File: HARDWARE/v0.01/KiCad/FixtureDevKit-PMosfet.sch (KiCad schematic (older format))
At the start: 56 parts, among them J63 FET_0, J64 FET_4, J65 FET_1, J66 FET_5, J67 FET_2, J68 FET_6, J69 FET_3, J70 FET_7, Q10 NTF2955T1G, Q11 NTF2955T1G, Q12 NTF2955T1G, Q5 NTF2955T1G, Q6 NTF2955T1G, Q7 NTF2955T1G, Q8 NTF2955T1G, Q9 NTF2955T1G

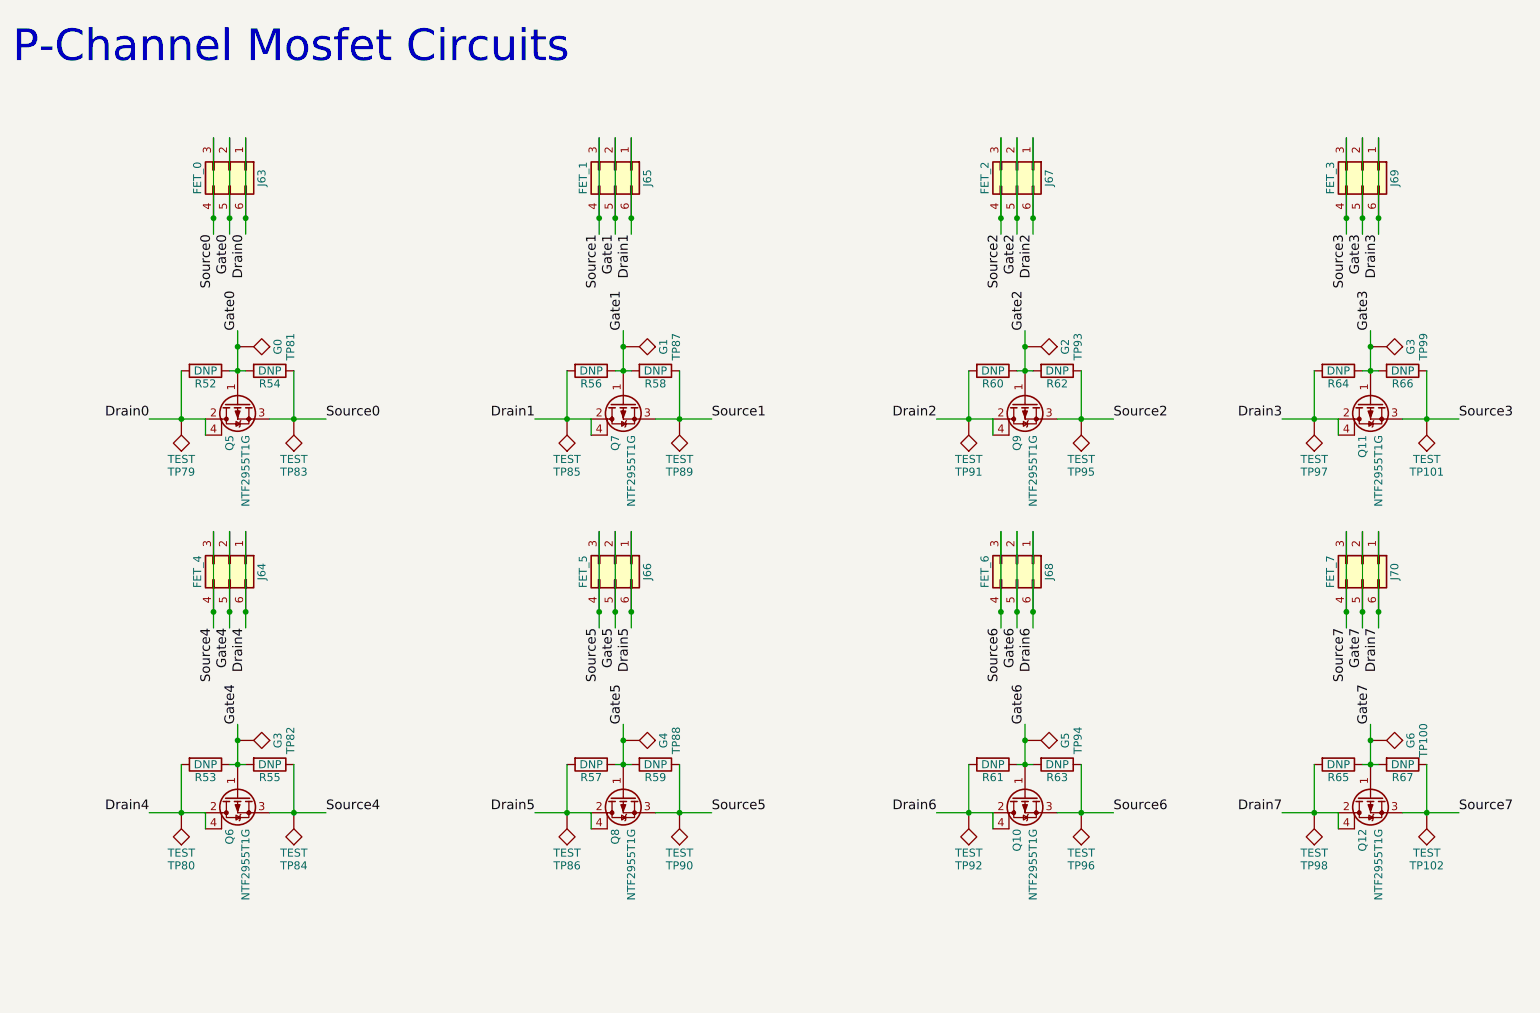
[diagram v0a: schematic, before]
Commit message: beginning pcb layout
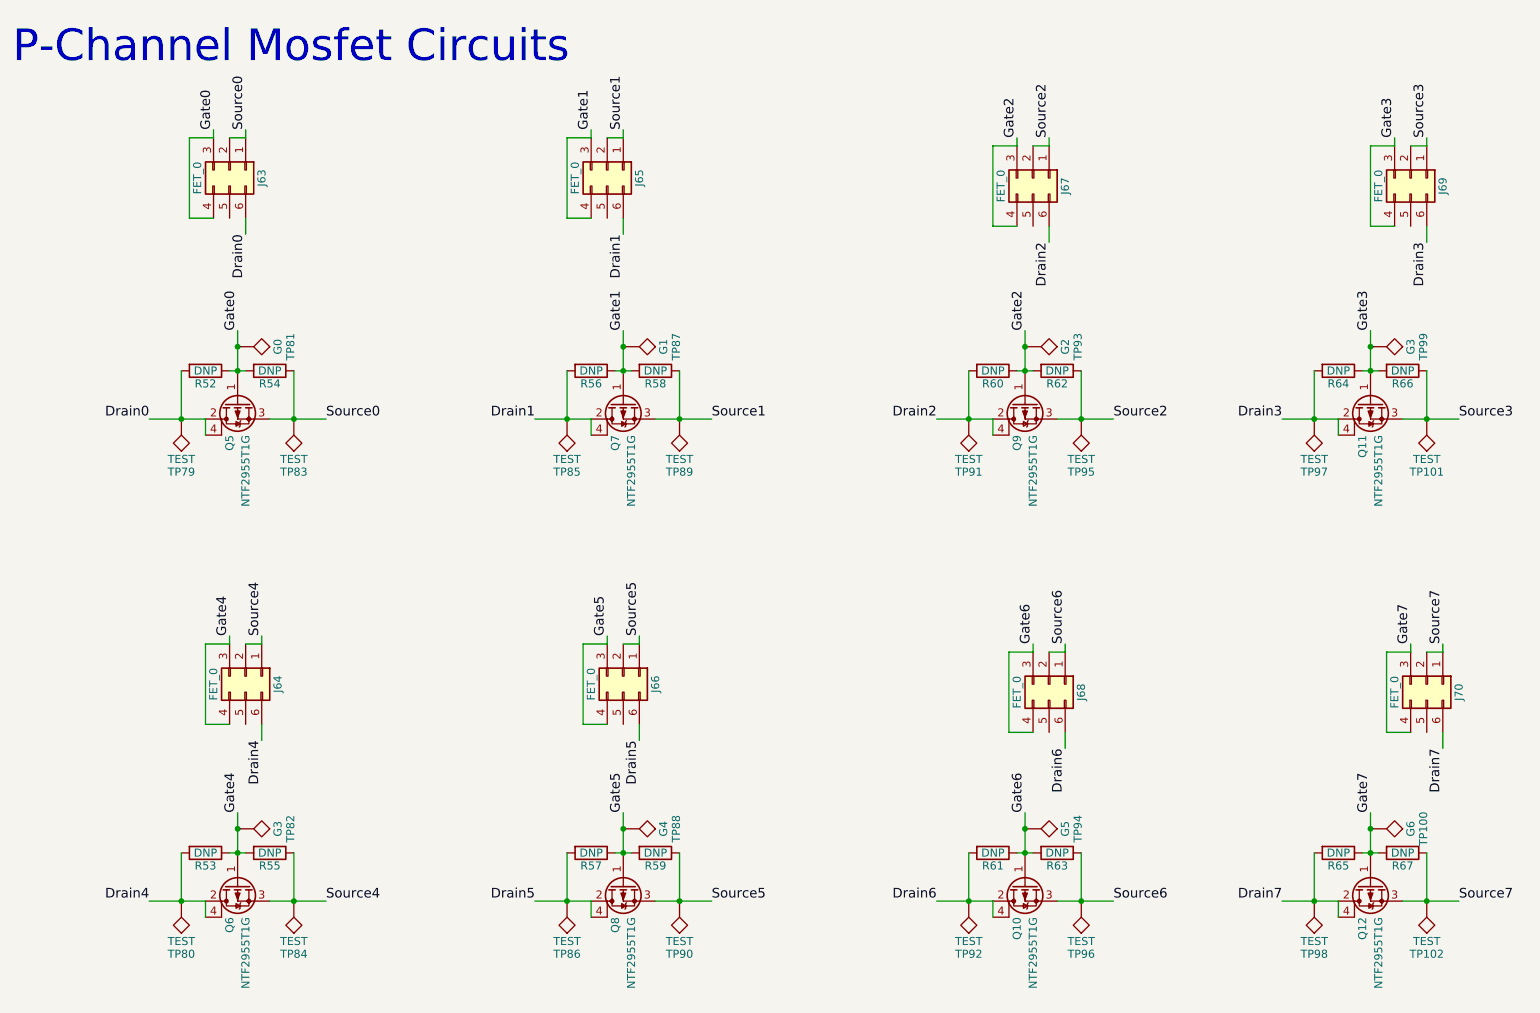
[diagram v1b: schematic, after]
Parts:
- J64: value FET_4 -> FET_0
- J65: value FET_1 -> FET_0
- J66: value FET_5 -> FET_0
- J67: value FET_2 -> FET_0
- J68: value FET_6 -> FET_0
- J69: value FET_3 -> FET_0
- J70: value FET_7 -> FET_0
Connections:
- net Drain0: no longer J63.1 (Pin_1)
- net Drain1: no longer J65.1 (Pin_1)
- net Drain2: no longer J67.1 (Pin_1)
- net Drain3: no longer J69.1 (Pin_1)
- net Drain4: no longer J64.1 (Pin_1)
- net Drain5: no longer J66.1 (Pin_1)
- net Drain6: no longer J68.1 (Pin_1)
- net Drain7: no longer J70.1 (Pin_1)
- net Gate0: now also J63.3 (Pin_3), J63.4 (Pin_4); no longer J63.2 (Pin_2), J63.5 (Pin_5)
- net Gate1: now also J65.3 (Pin_3), J65.4 (Pin_4); no longer J65.2 (Pin_2), J65.5 (Pin_5)
- net Gate2: now also J67.3 (Pin_3), J67.4 (Pin_4); no longer J67.2 (Pin_2), J67.5 (Pin_5)
- net Gate3: now also J69.3 (Pin_3), J69.4 (Pin_4); no longer J69.2 (Pin_2), J69.5 (Pin_5)
- net Gate4: now also J64.3 (Pin_3), J64.4 (Pin_4); no longer J64.2 (Pin_2), J64.5 (Pin_5)
- net Gate5: now also J66.3 (Pin_3), J66.4 (Pin_4); no longer J66.2 (Pin_2), J66.5 (Pin_5)
- net Gate6: now also J68.3 (Pin_3), J68.4 (Pin_4); no longer J68.2 (Pin_2), J68.5 (Pin_5)
- net Gate7: now also J70.3 (Pin_3), J70.4 (Pin_4); no longer J70.2 (Pin_2), J70.5 (Pin_5)
- net Source0: now also J63.1 (Pin_1), J63.2 (Pin_2); no longer J63.3 (Pin_3), J63.4 (Pin_4)
- net Source1: now also J65.1 (Pin_1), J65.2 (Pin_2); no longer J65.3 (Pin_3), J65.4 (Pin_4)
- net Source2: now also J67.1 (Pin_1), J67.2 (Pin_2); no longer J67.3 (Pin_3), J67.4 (Pin_4)
- net Source3: now also J69.1 (Pin_1), J69.2 (Pin_2); no longer J69.3 (Pin_3), J69.4 (Pin_4)
- net Source4: now also J64.1 (Pin_1), J64.2 (Pin_2); no longer J64.3 (Pin_3), J64.4 (Pin_4)
- net Source5: now also J66.1 (Pin_1), J66.2 (Pin_2); no longer J66.3 (Pin_3), J66.4 (Pin_4)
- net Source6: now also J68.1 (Pin_1), J68.2 (Pin_2); no longer J68.3 (Pin_3), J68.4 (Pin_4)
- net Source7: now also J70.1 (Pin_1), J70.2 (Pin_2); no longer J70.3 (Pin_3), J70.4 (Pin_4)
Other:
- moved on the sheet: Q10, Q12, Q6, Q8, R53, R55, R57, R59, R61, R63, R65, R67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
